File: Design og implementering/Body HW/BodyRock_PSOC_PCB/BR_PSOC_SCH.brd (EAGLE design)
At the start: 97.5 x 57.1 mm, 23 parts, among them T1 BC547, T2 BC547

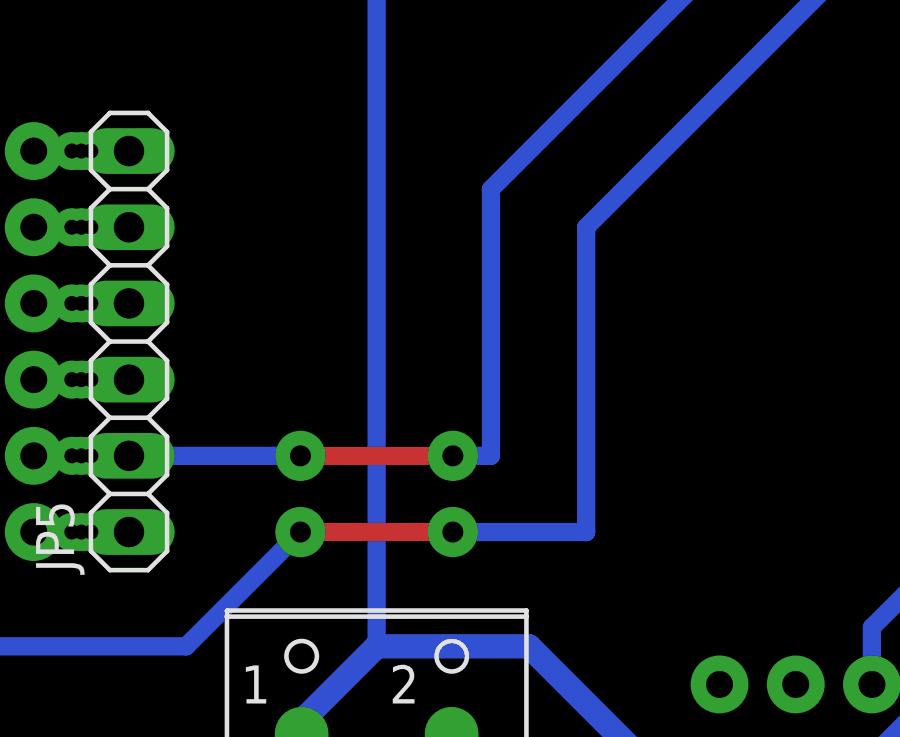
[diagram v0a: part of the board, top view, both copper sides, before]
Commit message: Added a section about the PSoC shield. -Felix
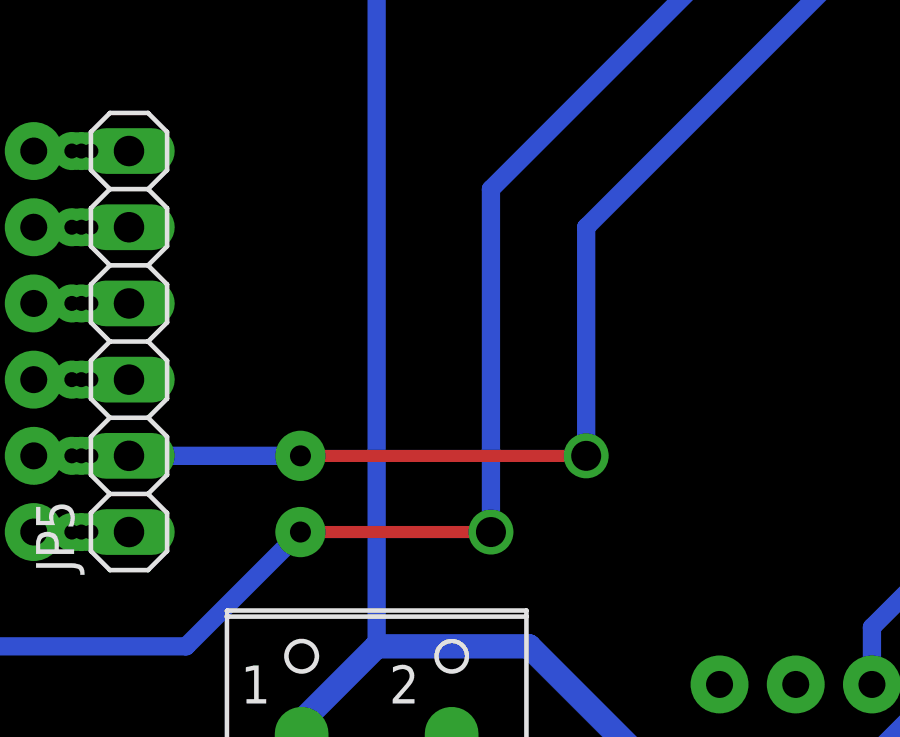
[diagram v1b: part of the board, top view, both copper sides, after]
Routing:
- net N$5: track 87.6 -> 90.1 mm
- net N$6: track 109.1 -> 106.6 mm
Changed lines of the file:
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@@
 <wire x1="8.89" y1="13.97" x2="17.78" y2="13.97" width="0.6096" layer="16"/>
 <via x="17.78" y="13.97" extent="1-16" drill="0.7" diameter="1.6764" shape="square"/>
-<wire x1="17.78" y1="13.97" x2="22.86" y2="13.97" width="0.6096" layer="1"/>
-<via x="22.86" y="13.97" extent="1-16" drill="0.7" diameter="1.6764" shape="square"/>
-<wire x1="22.86" y1="13.97" x2="24.13" y2="13.97" width="0.6096" layer="16"/>
-<wire x1="24.13" y1="13.97" x2="24.13" y2="22.86" width="0.6096" layer="16"/>
+<wire x1="17.78" y1="13.97" x2="22.86" y2="13.97" width="0" layer="19" extent="1-16"/>
+<wire x1="22.86" y1="13.97" x2="22.86" y2="13.97" width="0" layer="19" extent="1-16"/>
+<wire x1="24.13" y1="11.43" x2="24.13" y2="22.86" width="0.6096" layer="16"/>
 <wire x1="24.13" y1="22.86" x2="37.465" y2="36.195" width="0.6096" layer="16"/>
 <wire x1="37.465" y1="36.195" x2="56.515" y2="36.195" width="0.6096" layer="16"/>
@@
 <wire x1="63.8175" y1="48.5775" x2="64.77" y2="49.53" width="0.6096" layer="16"/>
 <wire x1="64.77" y1="49.53" x2="64.77" y2="50.8" width="0.6096" layer="16"/>
+<via x="24.13" y="11.43" extent="1-16" drill="1" shape="square"/>
+<wire x1="24.13" y1="11.43" x2="17.78" y2="11.43" width="0.4064" layer="1"/>
+<wire x1="17.78" y1="11.43" x2="17.78" y2="13.97" width="0" layer="19" extent="1-16"/>
 </signal>
 <signal name="N$6">
@@
 <wire x1="13.97" y1="7.62" x2="17.78" y2="11.43" width="0.6096" layer="16"/>
 <via x="17.78" y="11.43" extent="1-16" drill="0.7" diameter="1.6764" shape="square"/>
-<wire x1="17.78" y1="11.43" x2="22.86" y2="11.43" width="0.6096" layer="1"/>
-<via x="22.86" y="11.43" extent="1-16" drill="0.7" diameter="1.6764" shape="square"/>
-<wire x1="22.86" y1="11.43" x2="27.305" y2="11.43" width="0.6096" layer="16"/>
-<wire x1="27.305" y1="11.43" x2="27.305" y2="21.59" width="0.6096" layer="16"/>
+<wire x1="17.78" y1="11.43" x2="22.86" y2="11.43" width="0" layer="19" extent="1-16"/>
+<wire x1="22.86" y1="11.43" x2="22.86" y2="11.43" width="0" layer="19" extent="1-16"/>
+<wire x1="27.305" y1="13.97" x2="27.305" y2="21.59" width="0.6096" layer="16"/>
 <wire x1="27.305" y1="21.59" x2="38.735" y2="33.02" width="0.6096" layer="16"/>
 <wire x1="38.735" y1="33.02" x2="59.055" y2="33.02" width="0.6096" layer="16"/>
@@
 <wire x1="64.135" y1="46.355" x2="59.055" y2="46.355" width="0.6096" layer="16"/>
 <wire x1="59.055" y1="46.355" x2="59.055" y2="42.545" width="0.6096" layer="16"/>
+<via x="27.305" y="13.97" extent="1-16" drill="1" shape="square"/>
+<wire x1="27.305" y1="13.97" x2="17.78" y2="13.97" width="0.4064" layer="1"/>
+<wire x1="17.78" y1="13.97" x2="17.78" y2="11.43" width="0" layer="19" extent="1-16"/>
 </signal>
 <signal name="N$8">
